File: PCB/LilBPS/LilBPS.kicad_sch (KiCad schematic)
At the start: 45 parts, among them J1 Screw_Terminal_01x02, J2 Conn_01x02_Pin, J3 USB_C_Receptacle_PowerOnly_6P, P1 USB_C_Plug_USB2.0, Q1 DMP3013SFV, Q2 DMP3013SFV, SW1 SW_Push, SW2 SW_Push, U1 STUSB4500QTR, U2 AMS1117-3.3, U3 ESP32-C3-WROOM-02

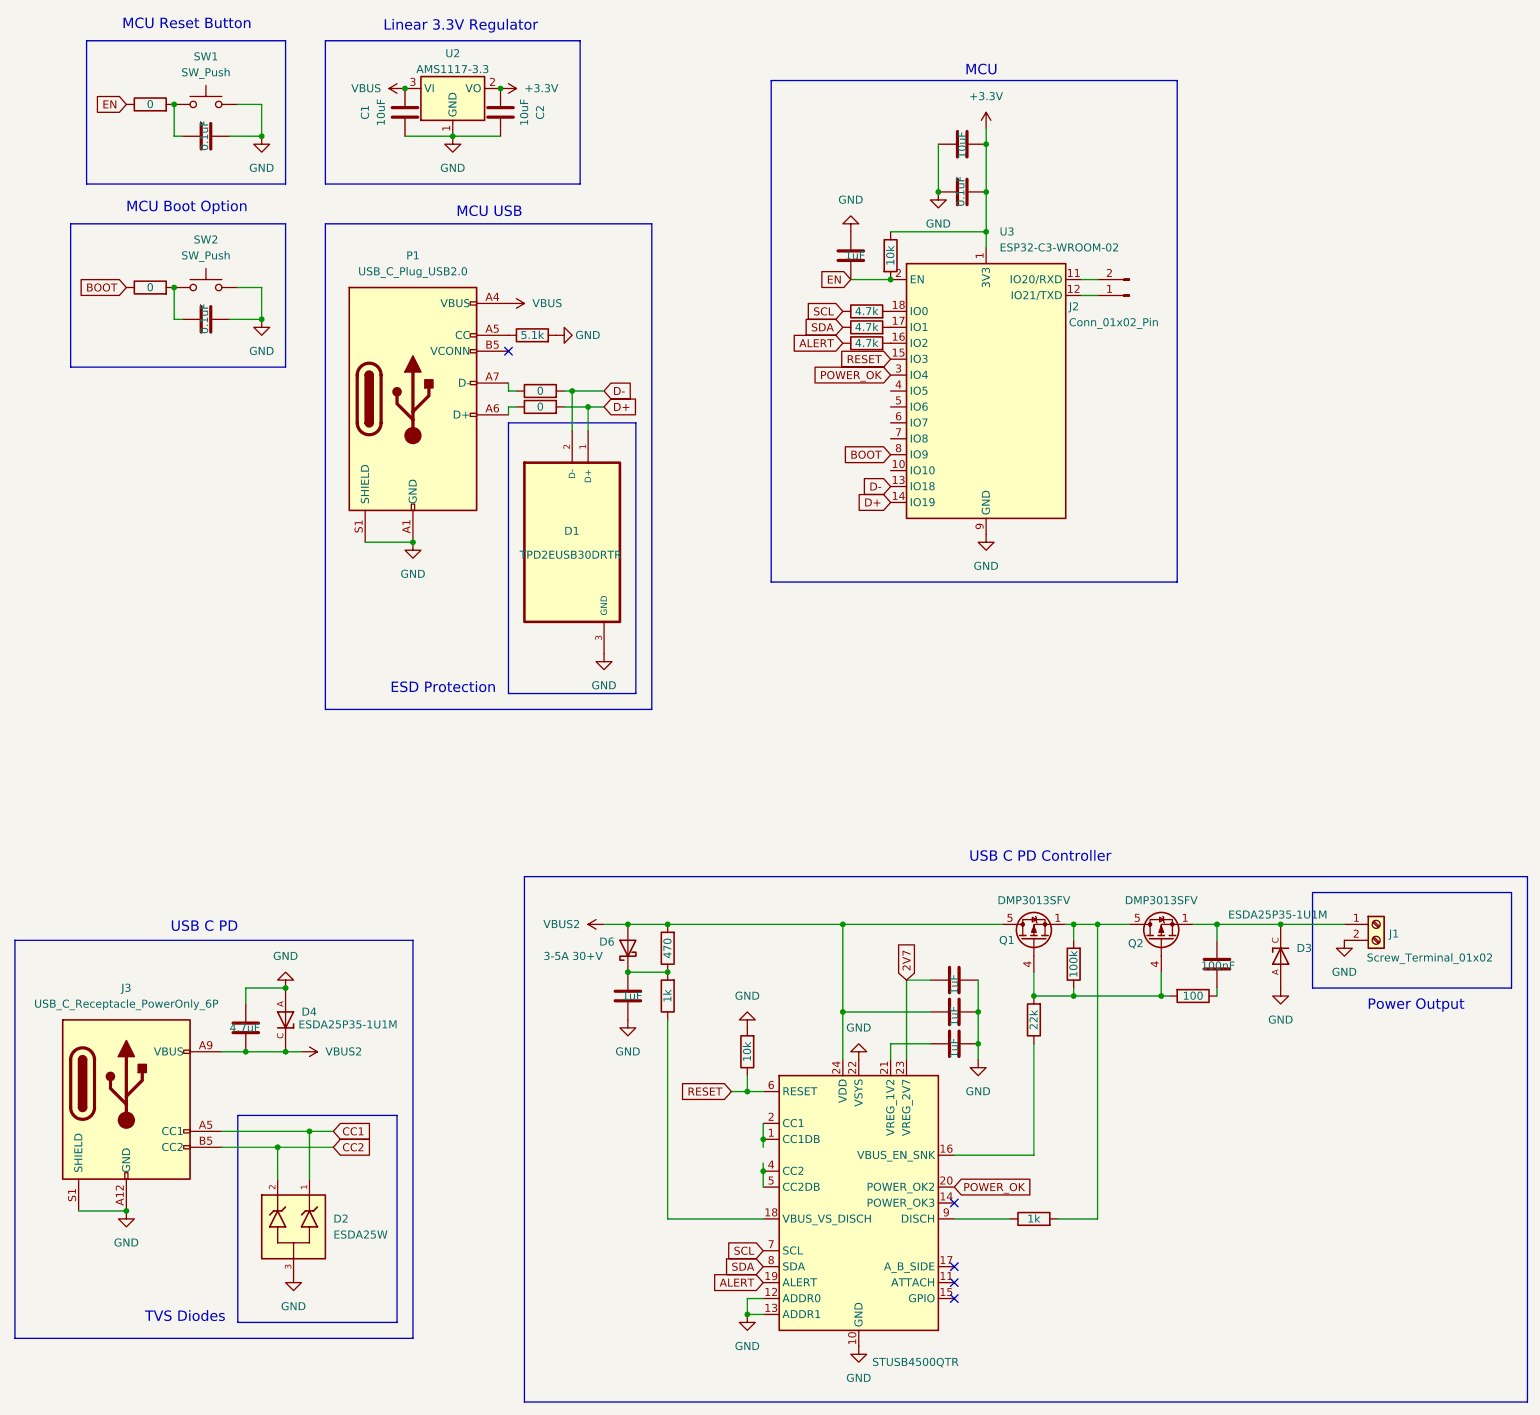
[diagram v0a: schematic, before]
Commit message: First journal entry :D
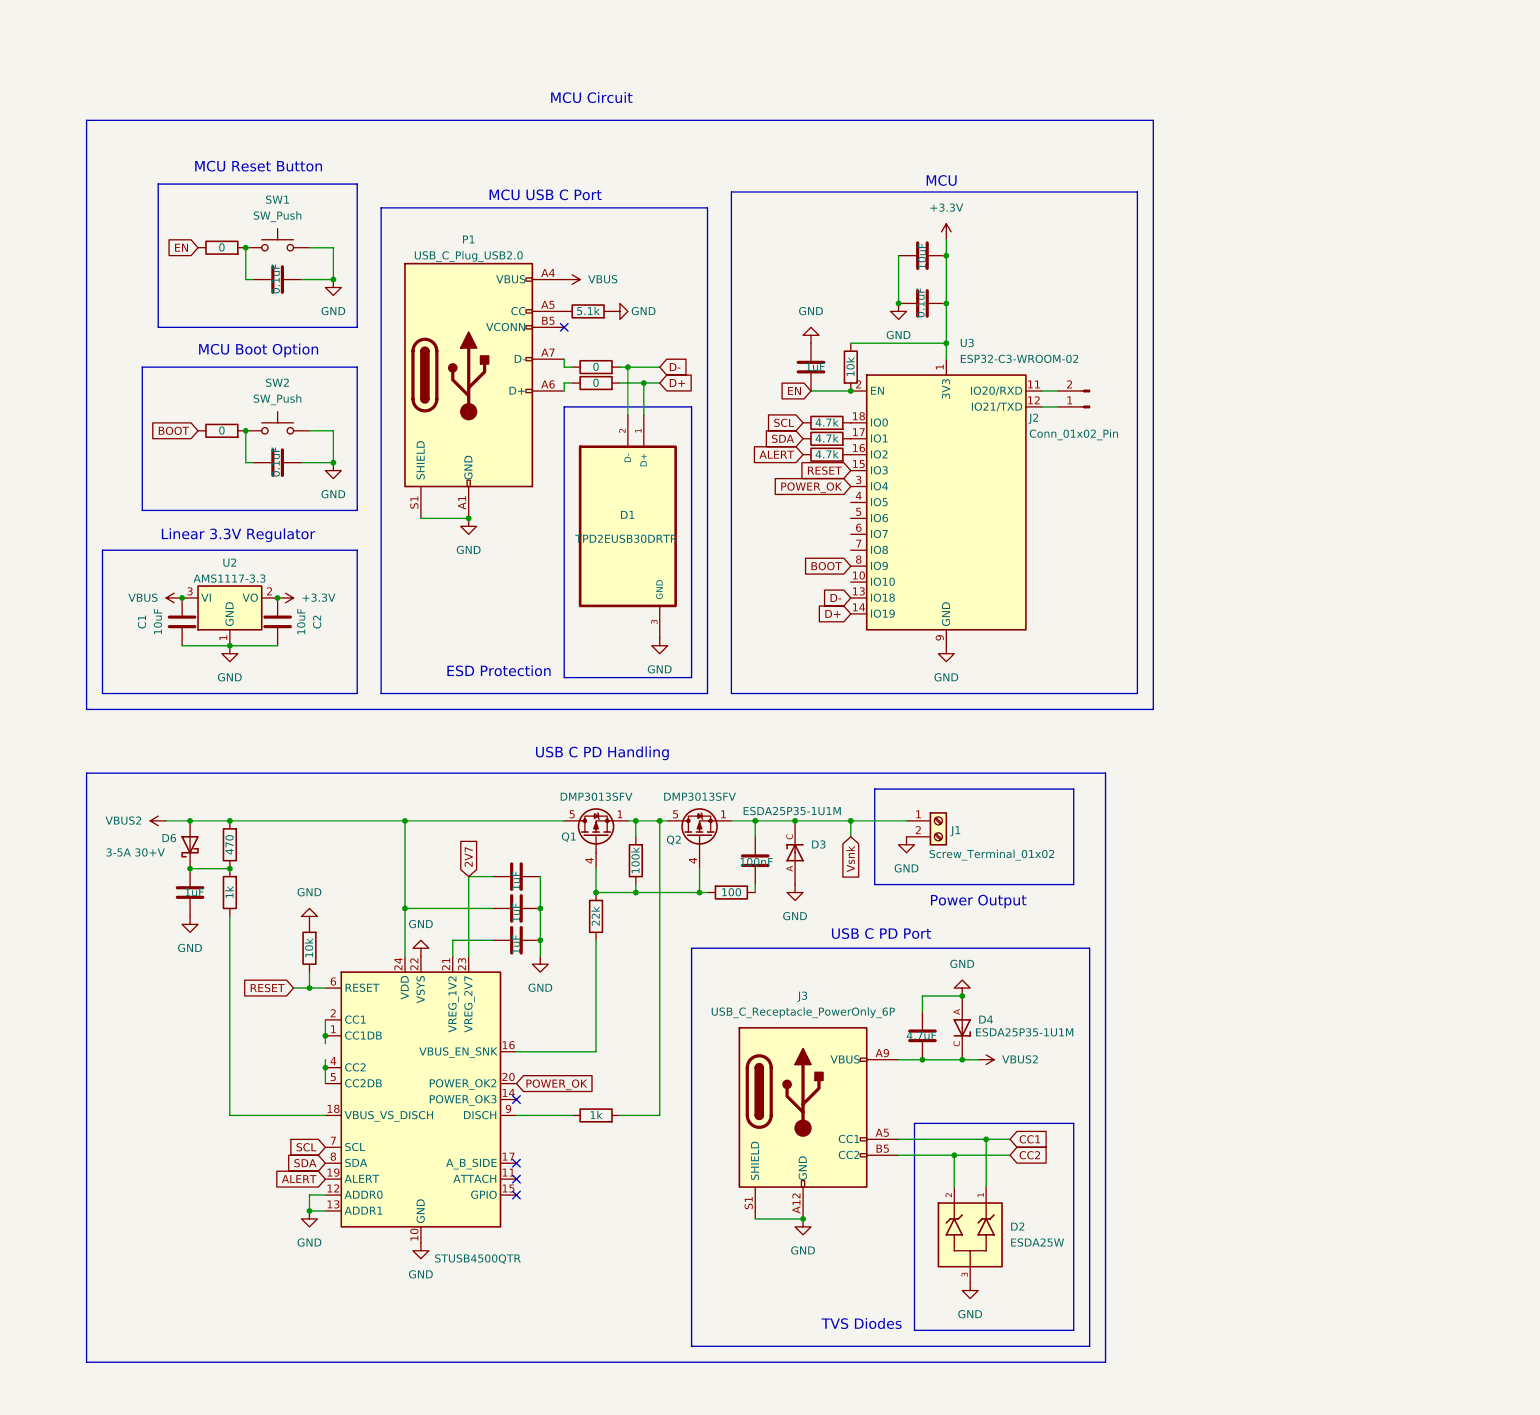
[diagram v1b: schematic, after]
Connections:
- net Vsnk: now reaches C11.1, D3.C, J1.1 (Pin_1), Q2.1 (S), Q2.2 (S), Q2.3 (S)
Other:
- note added: "MCU Circuit"
- note added: "MCU USB C Port"
- note added: "USB C PD Handling"
- note added: "USB C PD Port"
- note removed: "MCU USB"
- note removed: "USB C PD"
- note removed: "USB C PD Controller"
- moved on the sheet: C1, C2, D1, D2, D3, D4, D6, J1, J2, J3, P1, Q1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
